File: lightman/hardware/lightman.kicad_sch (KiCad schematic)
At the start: 42 parts, among them J1 Barrel_Jack_Switch, J2 Mini-DIN-6, J3 DE15_Socket_HighDensity_Mount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, J4 DE9_Pins, SW1 POWER, U1 LEVEL SHIFTER, U2 L7805, U3 MAX3232, U4 MAX3232, U5 MAX3232

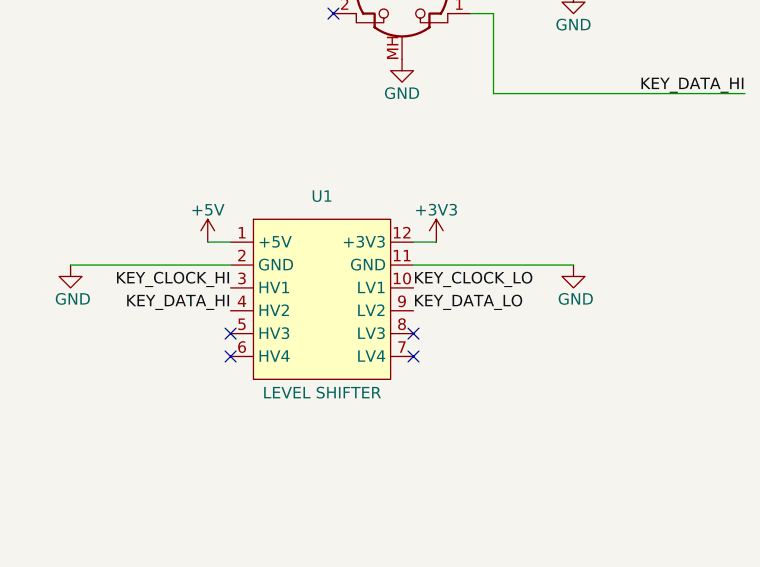
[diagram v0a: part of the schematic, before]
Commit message: lightman cleanup; more work pending
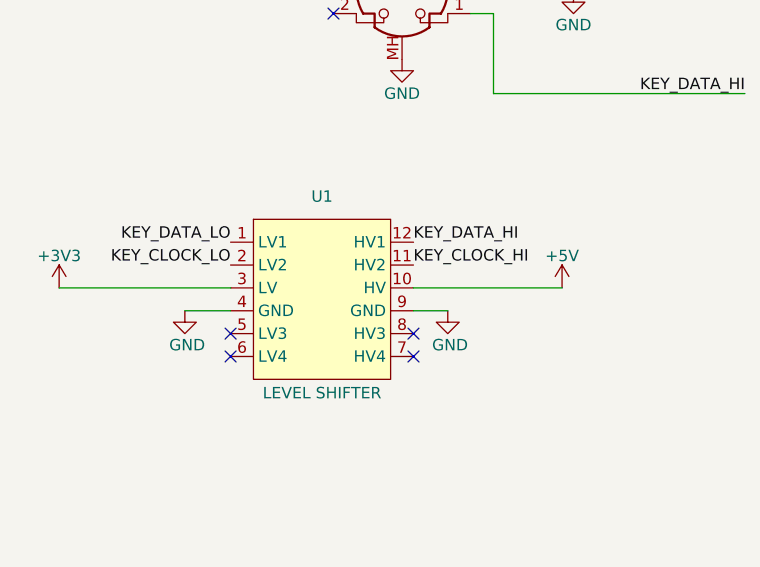
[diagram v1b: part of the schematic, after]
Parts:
- C2: footprint Capacitor_THT:CP_Radial_D6.3mm_P2.50mm -> Capacitor_THT:CP_Radial_D10.0mm_P5.00mm
- C3: footprint Capacitor_THT:CP_Radial_D5.0mm_P2.50mm -> Capacitor_THT:CP_Radial_D10.0mm_P5.00mm
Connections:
- net +3V3: now also U1.3 (LV); no longer U1.12 (+3V3)
- net +5V: now also U1.10 (HV); no longer U1.1 (+5V)
- net GND: now also U1.4 (GND), U1.9 (GND); no longer U1.11 (GND), U1.2 (GND)
- net KEY_CLOCK_HI: now also U1.11 (HV2); no longer U1.3 (HV1)
- net KEY_CLOCK_LO: now also U1.2 (LV2); no longer U1.10 (LV1)
- net KEY_DATA_HI: now also U1.12 (HV1); no longer U1.4 (HV2)
- net KEY_DATA_LO: now also U1.1 (LV1); no longer U1.9 (LV2)
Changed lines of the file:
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@@
 	(wire
 		(pts
-			(xy 26.67 166.37) (xy 44.45 166.37)
-		)
-		(stroke
-			(width 0)
-			(type default)
-		)
-	)
-	(wire
-		(pts
 			(xy 264.16 121.92) (xy 273.05 121.92)
 		)
@@
 	(wire
 		(pts
-			(xy 64.77 163.83) (xy 67.31 163.83)
-		)
-		(stroke
-			(width 0)
-			(type default)
-		)
-	)
-	(wire
-		(pts
 			(xy 30.48 118.11) (xy 180.34 118.11)
 		)
@@
 	(wire
 		(pts
+			(xy 64.77 171.45) (xy 68.58 171.45)
+		)
+		(stroke
+			(width 0)
+			(type default)
+		)
+	)
+	(wire
+		(pts
 			(xy 119.38 60.96) (xy 119.38 63.5)
 		)
@@
 	(wire
 		(pts
+			(xy 64.77 168.91) (xy 81.28 168.91)
+		)
+		(stroke
+			(width 0)
+			(type default)
+		)
+	)
+	(wire
+		(pts
 			(xy 106.68 237.49) (xy 113.03 237.49)
 		)
@@
 	(wire
 		(pts
-			(xy 64.77 166.37) (xy 82.55 166.37)
+			(xy 25.4 168.91) (xy 44.45 168.91)
 		)
 		(stroke
@@
 	(wire
 		(pts
-			(xy 212.09 121.92) (xy 223.52 121.92)
+			(xy 39.37 171.45) (xy 44.45 171.45)
 		)
 		(stroke
@@
 	(wire
 		(pts
-			(xy 41.91 163.83) (xy 44.45 163.83)
+			(xy 212.09 121.92) (xy 223.52 121.92)
 		)
 		(stroke
@@
 	)
 	(label "KEY_DATA_LO"
-		(at 64.77 171.45 0)
+		(at 44.45 163.83 180)
 		(effects
 			(font
 				(size 1.27 1.27)
 			)
-			(justify left bottom)
+			(justify right bottom)
 		)
 	)
@@
 	)
 	(label "KEY_DATA_HI"
-		(at 44.45 171.45 180)
+		(at 64.77 163.83 0)
 		(effects
 			(font
 				(size 1.27 1.27)
 			)
-			(justify right bottom)
+			(justify left bottom)
 		)
 	)
@@
 	)
 	(label "KEY_CLOCK_LO"
-		(at 64.77 168.91 0)
+		(at 44.45 166.37 180)
 		(effects
 			(font
 				(size 1.27 1.27)
 			)
-			(justify left bottom)
+			(justify right bottom)
 		)
 	)
 	(label "KEY_CLOCK_HI"
-		(at 44.45 168.91 180)
+		(at 64.77 166.37 0)
 		(effects
 			(font
 				(size 1.27 1.27)
 			)
-			(justify right bottom)
+			(justify left bottom)
 		)
 	)
@@
 	(symbol
 		(lib_id "power:+3V3")
-		(at 67.31 163.83 0)
+		(at 25.4 168.91 0)
 		(unit 1)
 		(body_style 1)
@@
 		(dnp no)
 		(property "Reference" "#PWR07"
-			(at 67.31 167.64 0)
+			(at 25.4 172.72 0)
 			(hide yes)
 			(show_name no)
@@
 		)
 		(property "Value" "+3V3"
-			(at 67.31 160.274 0)
+			(at 25.4 165.354 0)
 			(show_name no)
 			(do_not_autoplace no)
@@
 		)
 		(property "Footprint" ""
-			(at 67.31 163.83 0)
+			(at 25.4 168.91 0)
 			(hide yes)
 			(show_name no)
@@
 		)
 		(property "Datasheet" ""
-			(at 67.31 163.83 0)
+			(at 25.4 168.91 0)
 			(hide yes)
 			(show_name no)
@@
 		)
 		(property "Description" "Power symbol creates a global label with name \"+3V3\""
-			(at 67.31 163.83 0)
+			(at 25.4 168.91 0)
 			(hide yes)
 			(show_name no)
@@
 	(symbol
 		(lib_id "power:GND")
-		(at 82.55 166.37 0)
+		(at 68.58 171.45 0)
 		(unit 1)
 		(body_style 1)
@@
 		(dnp no)
 		(property "Reference" "#PWR012"
-			(at 82.55 172.72 0)
+			(at 68.58 177.8 0)
 			(hide yes)
 			(show_name no)
@@
 		)
 		(property "Value" "GND"
-			(at 82.804 170.18 0)
+			(at 68.834 175.26 0)
 			(show_name no)
 			(do_not_autoplace no)
@@
 		)
 		(property "Footprint" ""
-			(at 82.55 166.37 0)
+			(at 68.58 171.45 0)
 			(hide yes)
 			(show_name no)
@@
 		)
 		(property "Datasheet" ""
-			(at 82.55 166.37 0)
+			(at 68.58 171.45 0)
 			(hide yes)
 			(show_name no)
@@
 		)
 		(property "Description" "Power symbol creates a global label with name \"GND\" , ground"
-			(at 82.55 166.37 0)
+			(at 68.58 171.45 0)
 			(hide yes)
 			(show_name no)
@@
 			)
 		)
-		(property "Footprint" "Capacitor_THT:CP_Radial_D6.3mm_P2.50mm"
+		(property "Footprint" "Capacitor_THT:CP_Radial_D10.0mm_P5.00mm"
 			(at 120.3452 247.65 0)
 			(hide yes)
@@
 	(symbol
 		(lib_id "power:+5V")
-		(at 41.91 163.83 0)
+		(at 81.28 168.91 0)
 		(unit 1)
 		(body_style 1)
@@
 		(dnp no)
 		(property "Reference" "#PWR03"
-			(at 41.91 167.64 0)
+			(at 81.28 172.72 0)
 			(hide yes)
 			(show_name no)
@@
 		)
 		(property "Value" "+5V"
-			(at 41.91 160.274 0)
+			(at 81.28 165.354 0)
 			(show_name no)
 			(do_not_autoplace no)
@@
 		)
 		(property "Footprint" ""
-			(at 41.91 163.83 0)
+			(at 81.28 168.91 0)
 			(hide yes)
 			(show_name no)
@@
 		)
 		(property "Datasheet" ""
-			(at 41.91 163.83 0)
+			(at 81.28 168.91 0)
 			(hide yes)
 			(show_name no)
@@
 		)
 		(property "Description" "Power symbol creates a global label with name \"+5V\""
-			(at 41.91 163.83 0)
+			(at 81.28 168.91 0)
 			(hide yes)
 			(show_name no)
@@
 	(symbol
 		(lib_id "power:GND")
-		(at 26.67 166.37 0)
+		(at 39.37 171.45 0)
 		(unit 1)
 		(body_style 1)
@@
 		(dnp no)
 		(property "Reference" "#PWR01"
-			(at 26.67 172.72 0)
+			(at 39.37 177.8 0)
 			(hide yes)
 			(show_name no)
@@
 		)
 		(property "Value" "GND"
-			(at 26.924 170.18 0)
+			(at 39.624 175.26 0)
 			(show_name no)
 			(do_not_autoplace no)
@@
 		)
 		(property "Footprint" ""
-			(at 26.67 166.37 0)
+			(at 39.37 171.45 0)
 			(hide yes)
 			(show_name no)
@@
 		)
 		(property "Datasheet" ""
-			(at 26.67 166.37 0)
+			(at 39.37 171.45 0)
 			(hide yes)
 			(show_name no)
@@
 		)
 		(property "Description" "Power symbol creates a global label with name \"GND\" , ground"
-			(at 26.67 166.37 0)
+			(at 39.37 171.45 0)
 			(hide yes)
 			(show_name no)
@@
 			)
 		)
-		(property "Footprint" "Capacitor_THT:CP_Radial_D5.0mm_P2.50mm"
+		(property "Footprint" "Capacitor_THT:CP_Radial_D10.0mm_P5.00mm"
 			(at 145.7452 247.65 0)
 			(hide yes)
